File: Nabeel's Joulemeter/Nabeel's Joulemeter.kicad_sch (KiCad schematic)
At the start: 16 parts, among them J1 XT60-M, J2 XT60-M, J3 22035035, U1 INA181A1QDBVRQ1, U2 PADS131M04QPWRQ1, U3 UA78M05QDCYRG4Q1

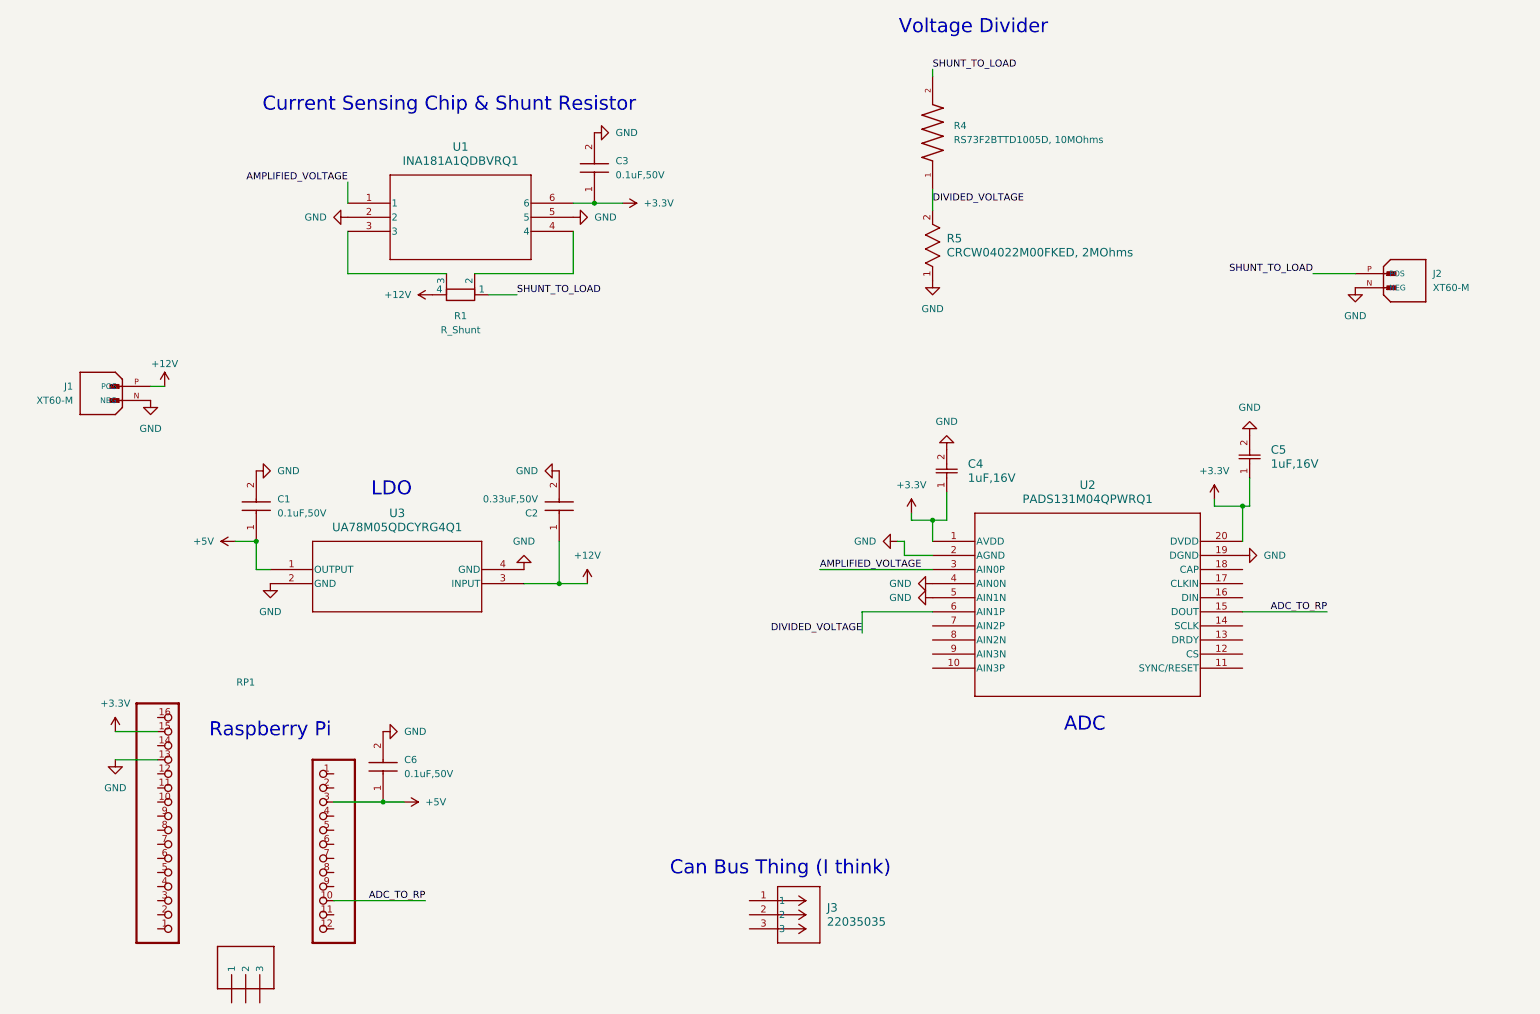
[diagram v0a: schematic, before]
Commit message: my board after grinding some more
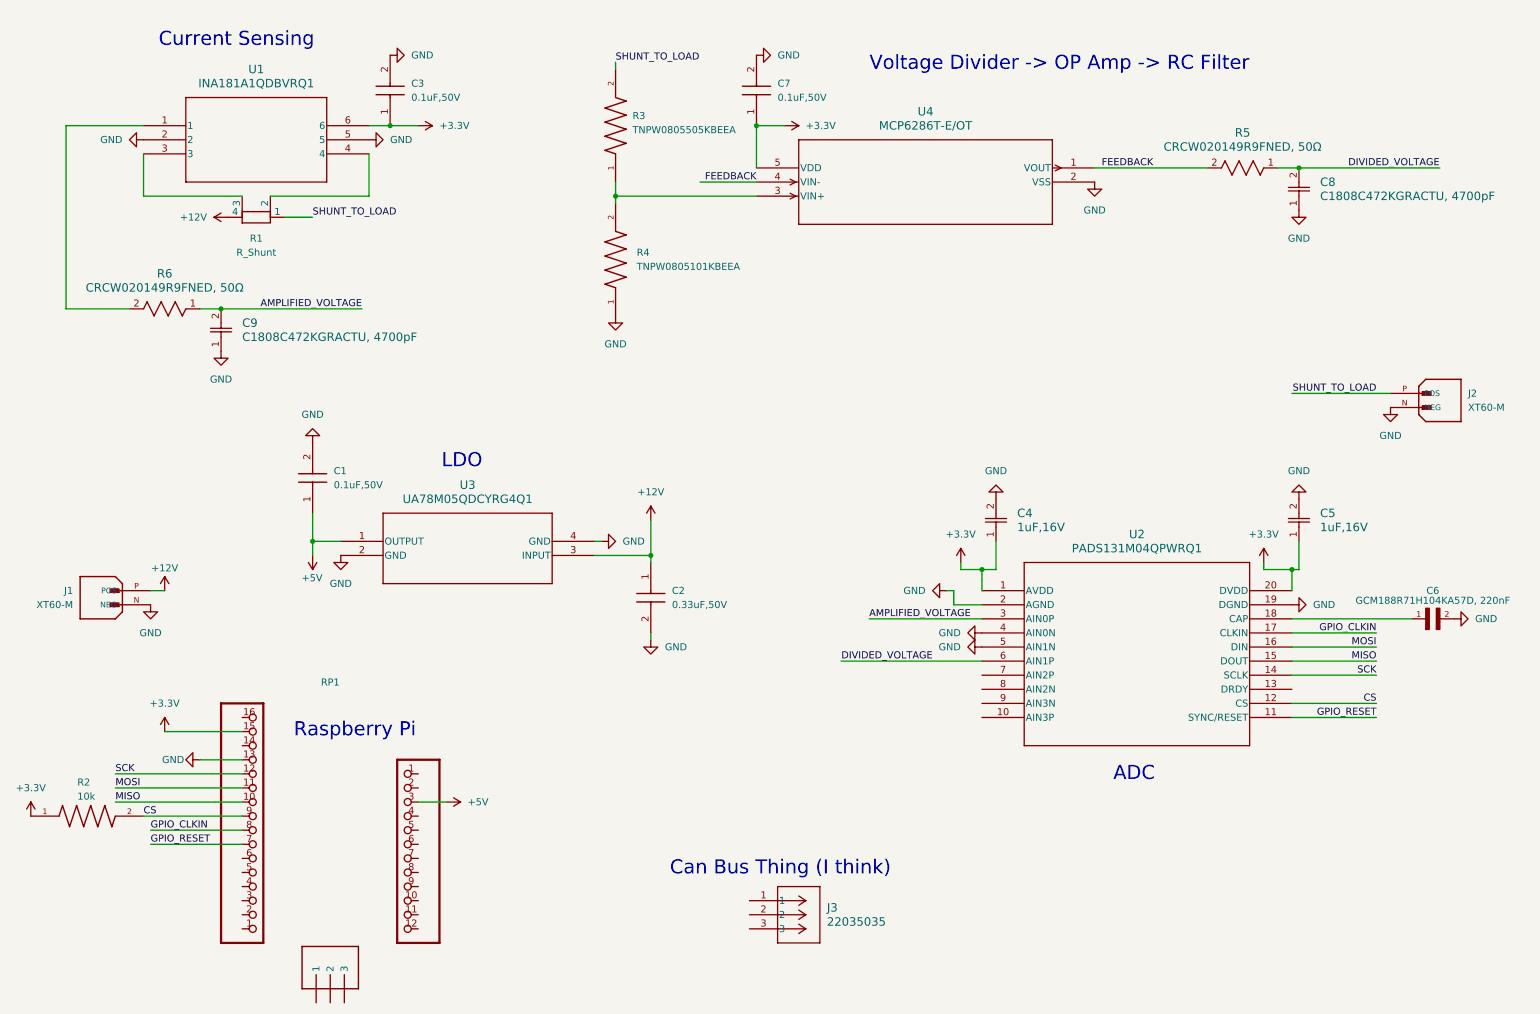
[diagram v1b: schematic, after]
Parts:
- removed C6: 0.1uF,50V, SMV_Passives:Cap0805, symbol SMV_Custom:C0805C104K5RACTU
- removed R4: RS73F2BTTD1005D, 10MOhms, RS73F2BTTD1005D:RESC3216X70N, symbol SMV_Custom:RS73F2BTTD1005D
- removed R5: CRCW04022M00FKED, 2MOhms, RES_CRCW_0402, symbol SMV_Custom:CRCW04022M00FKED
- added C6: GCM188R71H104KA57D, 220nF, SMV_Passives:0805RESC2012X60N, symbol SMV_Custom:GCM188R71H104KA57D
- added C7: 0.1uF,50V, SMV_Passives:Cap0805, symbol SMV_Custom:C0805C104K5RACTU
- added C8, C9: C1808C472KGRACTU, 4700pF, CAPC520220_215N_KEM, symbol SMV_Custom:C1808C472KGRACTU
- added R2: 10k, SMV_Passives:0805RESC2012X60N, symbol SMV_Custom:CRCW080510K0FKEAC
- added R3: TNPW0805505KBEEA, TNPW0805505KBEEA:RESC2012X55N, symbol SMV_Custom:TNPW0805505KBEEA
- added R4: TNPW0805101KBEEA, TNPW0805101KBEEA:RESC2012X55N, symbol SMV_Custom:TNPW0805101KBEEA
- added R5, R6: CRCW020149R9FNED, 50Ω, SMV_Passives:0805RESC2012X60N, symbol SMV_Custom:CRCW020149R9FNED
- added U4: MCP6286T-E/OT, SMV_ICs:SOT-23-5_MC_MCH, symbol SMV_Custom:MCP6286T-E_OT
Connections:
- net ADC_TO_RP is gone; now on net MISO: RP1.10, U2.15 (DOUT)
- net +3.3V: now also C7.1, R2.1, U4.5 (VDD)
- net AMPLIFIED_VOLTAGE: now also C9.2, R6.1; no longer U1.1
- net DIVIDED_VOLTAGE: now also C8.2, R5.1
- net GND: now also C6.2, C7.2, C8.1, C9.1, R4.1, U4.2 (VSS)
- net SHUNT_TO_LOAD: now also R3.2
- net GPIO_RESET: now reaches U2.11 (SYNC/RESET)
- net GPIO_RESET: now also RP1.7
- net CS: now reaches U2.12 (CS)
- net CS: now also RP1.9, R2.2
- net SCK: now reaches U2.14 (SCLK)
- net SCK: now also RP1.12
- net MOSI: now reaches U2.16 (DIN)
- net MOSI: now also RP1.11
- net GPIO_CLKIN: now reaches U2.17 (CLKIN)
- net GPIO_CLKIN: now also RP1.8
- net at U2.18 (CAP): now also C6.1
- net MISO: now reaches RP1.10
- new net: R3.1, R4.2, U4.3 (VIN+)
- new net: R6.2, U1.1
- new net FEEDBACK: R5.2, U4.1 (VOUT), U4.4 (VIN-)
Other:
- note added: "Current Sensing"
- note added: "Voltage Divider -> OP Amp -> RC Filter"
- note removed: "Current Sensing Chip & Shunt Resistor"
- note removed: "Voltage Divider"
- moved on the sheet: C1, C2, C3, C4, C5, J1, J2, R1, RP1, U1, U2, U3
